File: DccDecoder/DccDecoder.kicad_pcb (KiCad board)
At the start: 2 copper layers, 88.9 x 33 mm, 0 parts

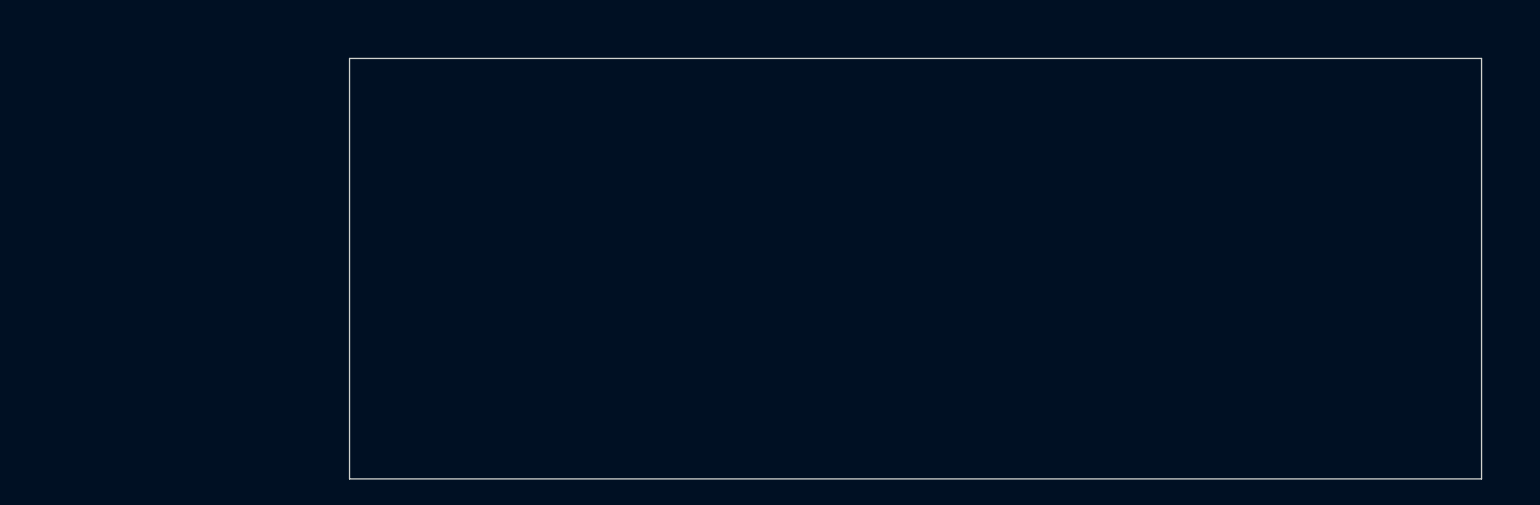
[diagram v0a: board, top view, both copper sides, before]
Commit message: 20:57 Titan.local
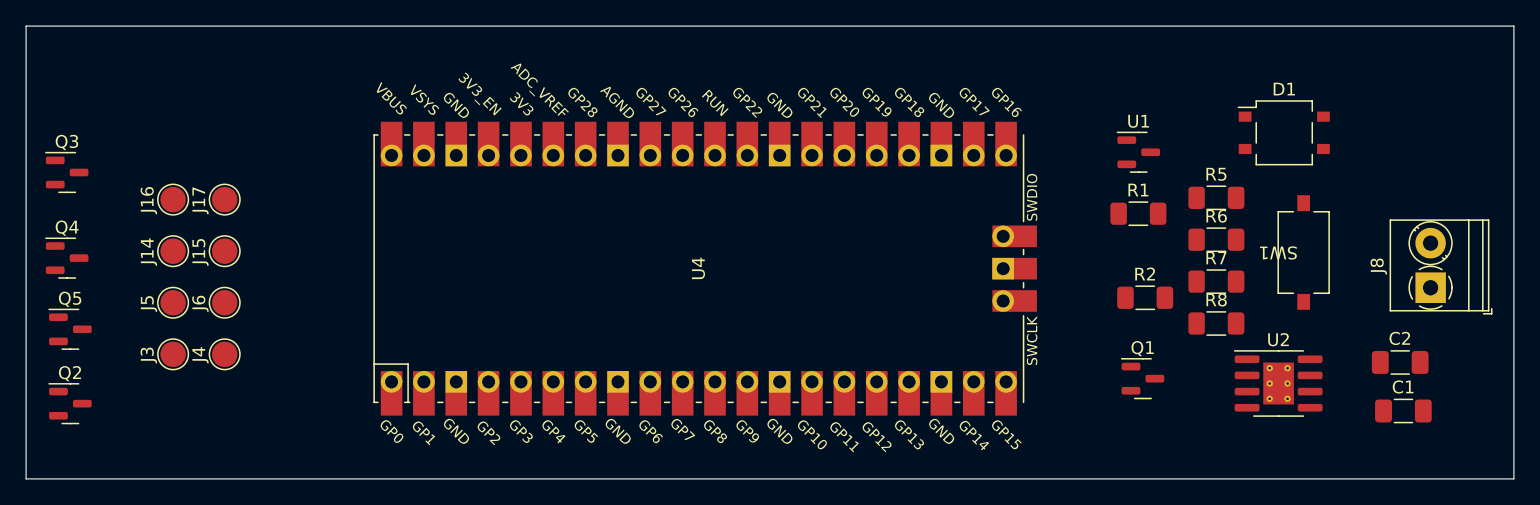
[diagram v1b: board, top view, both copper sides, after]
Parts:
- added C1: 10u, Capacitor_SMD:C_1206_3216Metric_Pad1.33x1.80mm_HandSolder, F.Cu at (184.4, 78.5)
- added C2: 10u, Capacitor_SMD:C_1206_3216Metric_Pad1.33x1.80mm_HandSolder, F.Cu at (184.1, 74.7)
- added D1: KMB24F, Package_TO_SOT_SMD:TO-269AA, F.Cu at (175.0, 56.6)
- added J14: +V, TestPoint:TestPoint_Pad_D2.0mm, F.Cu at (87.7, 65.9)
- added J15: M_OUT_B, TestPoint:TestPoint_Pad_D2.0mm, F.Cu at (91.8, 65.9)
- added J16: M_OUT_A, TestPoint:TestPoint_Pad_D2.0mm, F.Cu at (87.7, 61.9)
- added J17: GND, TestPoint:TestPoint_Pad_D2.0mm, F.Cu at (91.8, 61.9)
- added J3: 0, TestPoint:TestPoint_Pad_D2.0mm, F.Cu at (87.7, 74.0)
- added J4: 1, TestPoint:TestPoint_Pad_D2.0mm, F.Cu at (91.8, 74.0)
- added J5: 2, TestPoint:TestPoint_Pad_D2.0mm, F.Cu at (87.7, 70.0)
- added J6: 3, TestPoint:TestPoint_Pad_D2.0mm, F.Cu at (91.8, 70.0)
- added J8: DCC, TerminalBlock_Phoenix:TerminalBlock_Phoenix_PT-1,5-2-3.5-H_1x02_P3.50mm_Horizontal, F.Cu at (186.5, 68.8)
- added Q1: T2N7002BK, Package_TO_SOT_SMD:SOT-23, F.Cu at (163.9, 75.9)
- added Q2: T2N7002BK, Package_TO_SOT_SMD:SOT-23, F.Cu at (79.7, 77.9)
- added Q3: T2N7002BK, Package_TO_SOT_SMD:SOT-23, F.Cu at (79.4, 59.8)
- added Q4: T2N7002BK, Package_TO_SOT_SMD:SOT-23, F.Cu at (79.4, 66.5)
- added Q5: T2N7002BK, Package_TO_SOT_SMD:SOT-23, F.Cu at (79.7, 72.1)
- added R1: 6k8, Resistor_SMD:R_1206_3216Metric_Pad1.30x1.75mm_HandSolder, F.Cu at (163.6, 63.0)
- added R2: 6k8, Resistor_SMD:R_1206_3216Metric_Pad1.30x1.75mm_HandSolder, F.Cu at (164.1, 69.6)
- added R5: 6k8, Resistor_SMD:R_1206_3216Metric_Pad1.30x1.75mm_HandSolder, F.Cu at (169.7, 61.7)
- added R6: 6k8, Resistor_SMD:R_1206_3216Metric_Pad1.30x1.75mm_HandSolder, F.Cu at (169.7, 65.0)
- added R7: 1k, Resistor_SMD:R_1206_3216Metric_Pad1.30x1.75mm_HandSolder, F.Cu at (169.7, 68.3)
- added R8: 1k, Resistor_SMD:R_1206_3216Metric_Pad1.30x1.75mm_HandSolder, F.Cu at (169.7, 71.6)
- added SW1: SW_Push, Button_Switch_SMD:SW_Tactile_SPST_NO_Straight_CK_PTS636Sx25SMTRLFS, F.Cu at (176.5, 66.0)
- added U1: HT7533S, Package_TO_SOT_SMD:SOT-23, F.Cu at (163.6, 58.2)
- added U2: BDR6133, Package_SO:SOIC-8-1EP_3.9x4.9mm_P1.27mm_EP2.41x3.3mm_ThermalVias, F.Cu at (174.6, 76.3)
- added U4: Pico, MCU_RaspberryPi_and_Boards:RP2040Pico, F.Cu at (129.0, 67.3)
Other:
- board size 88.9 x 33 mm -> 116.8 x 35.6 mm
